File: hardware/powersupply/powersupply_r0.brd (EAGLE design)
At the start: 160 x 100 mm, 22 parts, among them CN17 22-23-2041

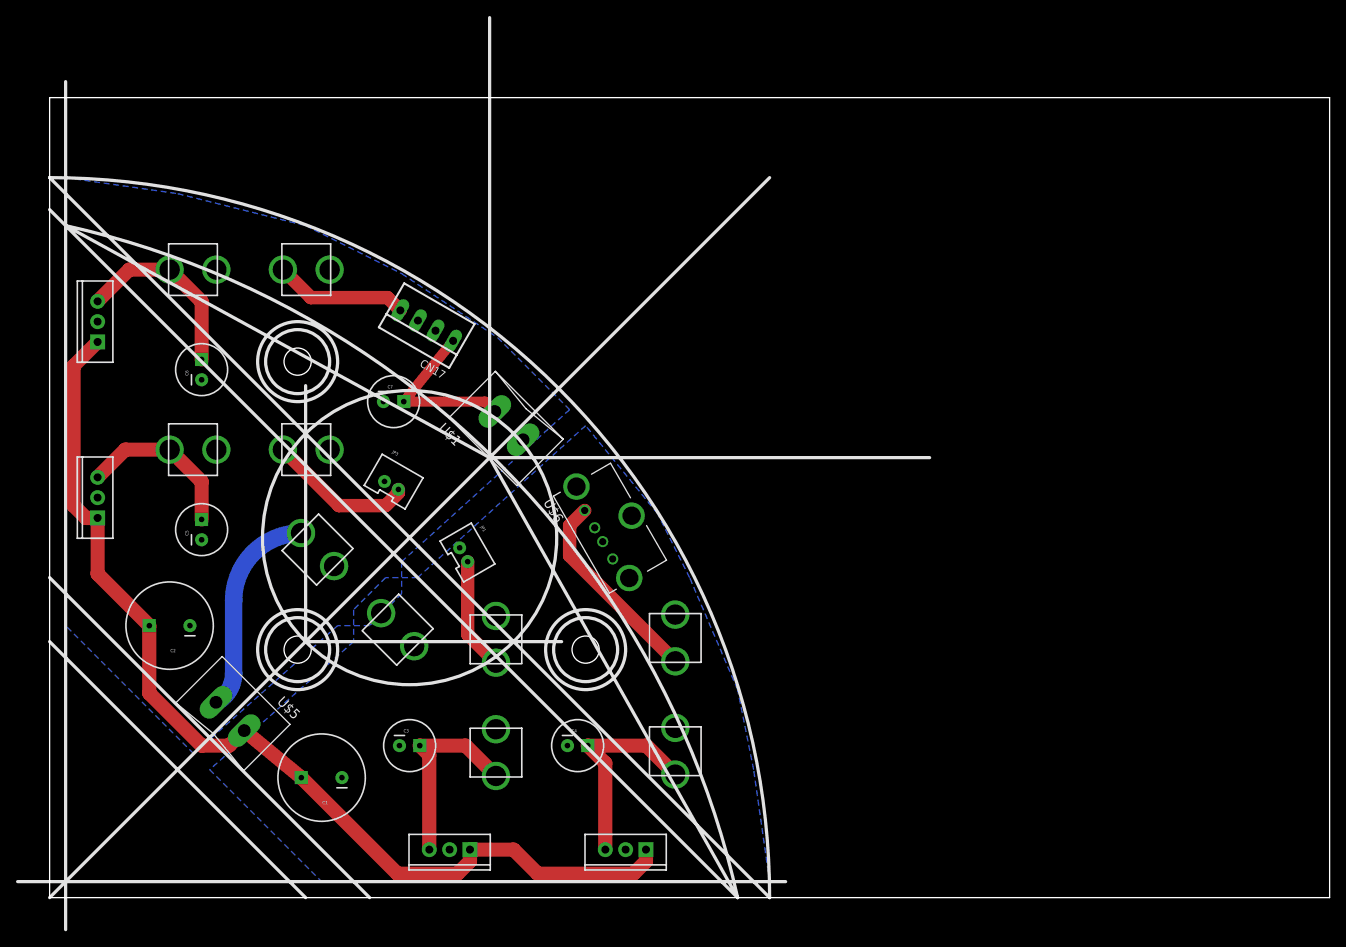
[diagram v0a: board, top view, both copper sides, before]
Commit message: cleanup and silkscreen
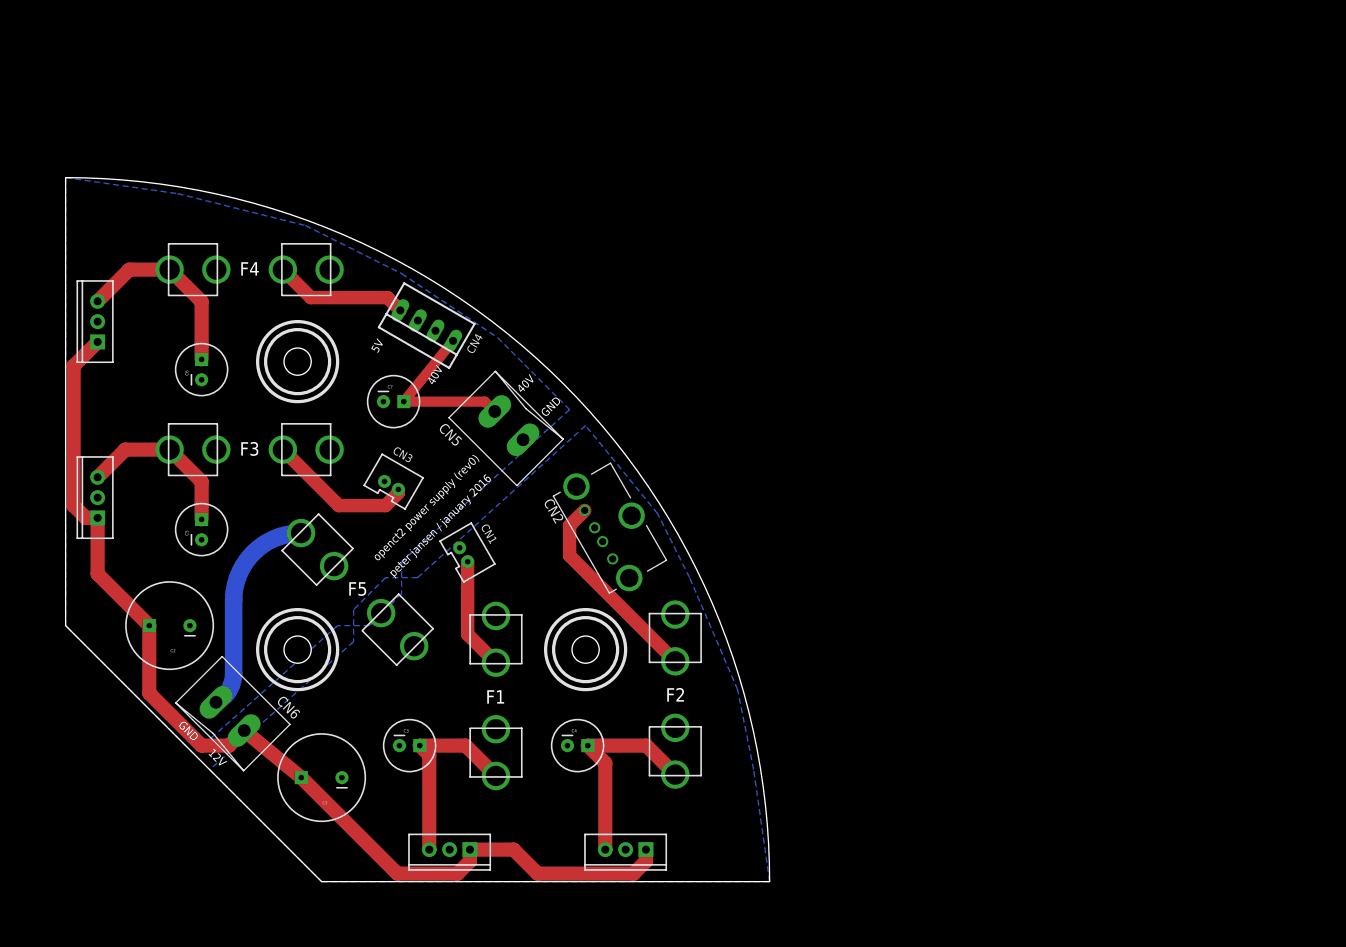
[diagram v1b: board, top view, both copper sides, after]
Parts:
- renumbered CN17 to CN4, JP1 to CN1, JP3 to CN3, U$1 to CN5, U$5 to CN6, U$6 to CN2
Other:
- board size 160 x 100 mm -> 88 x 88 mm
- board text added: "12V"
- board text added: "40V"
- board text added: "5V"
- board text added: "F1"
- board text added: "F2"
- board text added: "F3"
- board text added: "F4"
- board text added: "F5"
- board text added: "GND"
- board text added: "openct2 power supply (rev0)"
- board text added: "peter jansen / january 2016"
